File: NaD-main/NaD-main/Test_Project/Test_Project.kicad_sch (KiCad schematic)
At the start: 35 parts, among them J1 SWD, J2 USART1, J3 3V3, J5 Screw_Terminal_01x02, U1 AMS1117-3.3, U2 STM32F103C8Tx, U3 L298HN, U4 L7805, Y1 16 MHz

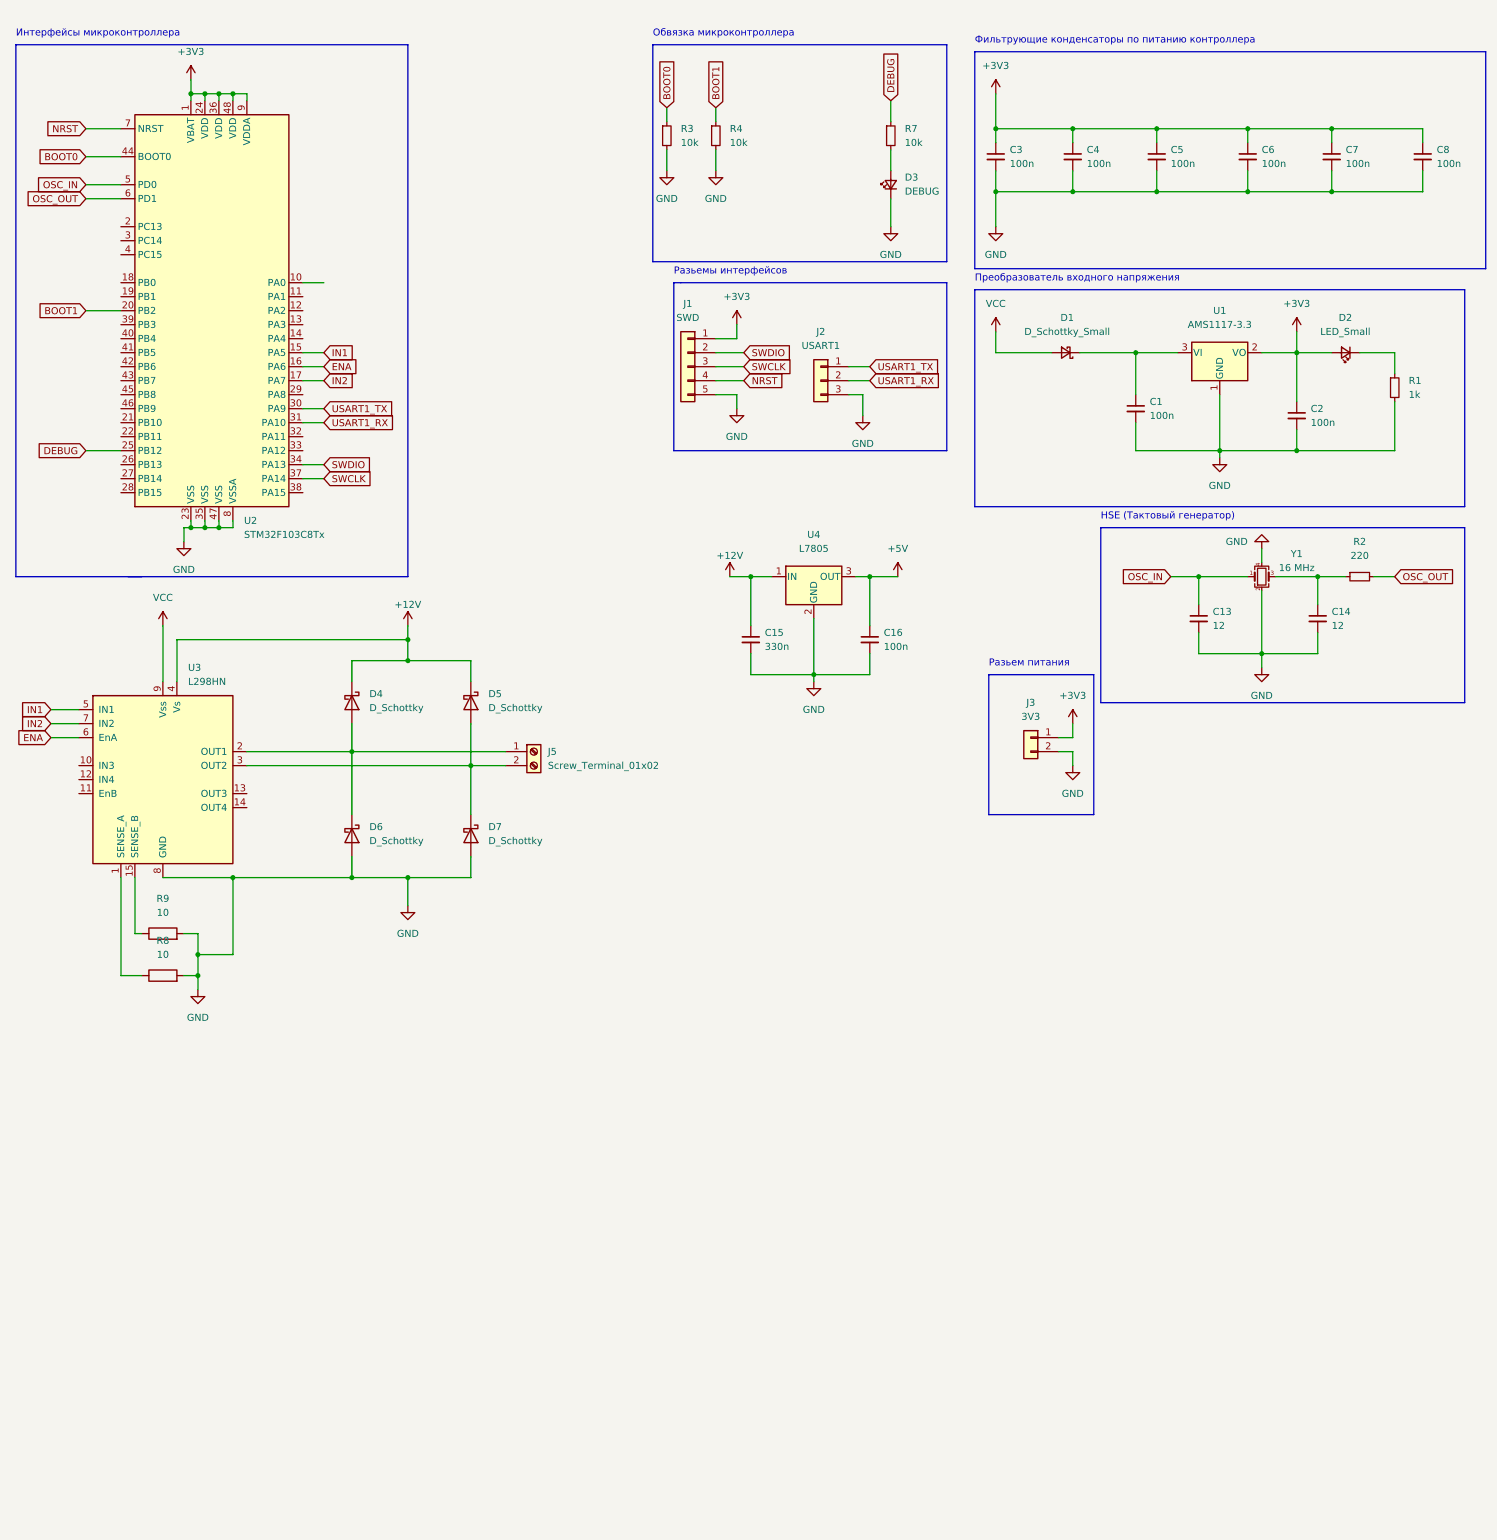
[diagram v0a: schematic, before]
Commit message: Documentation
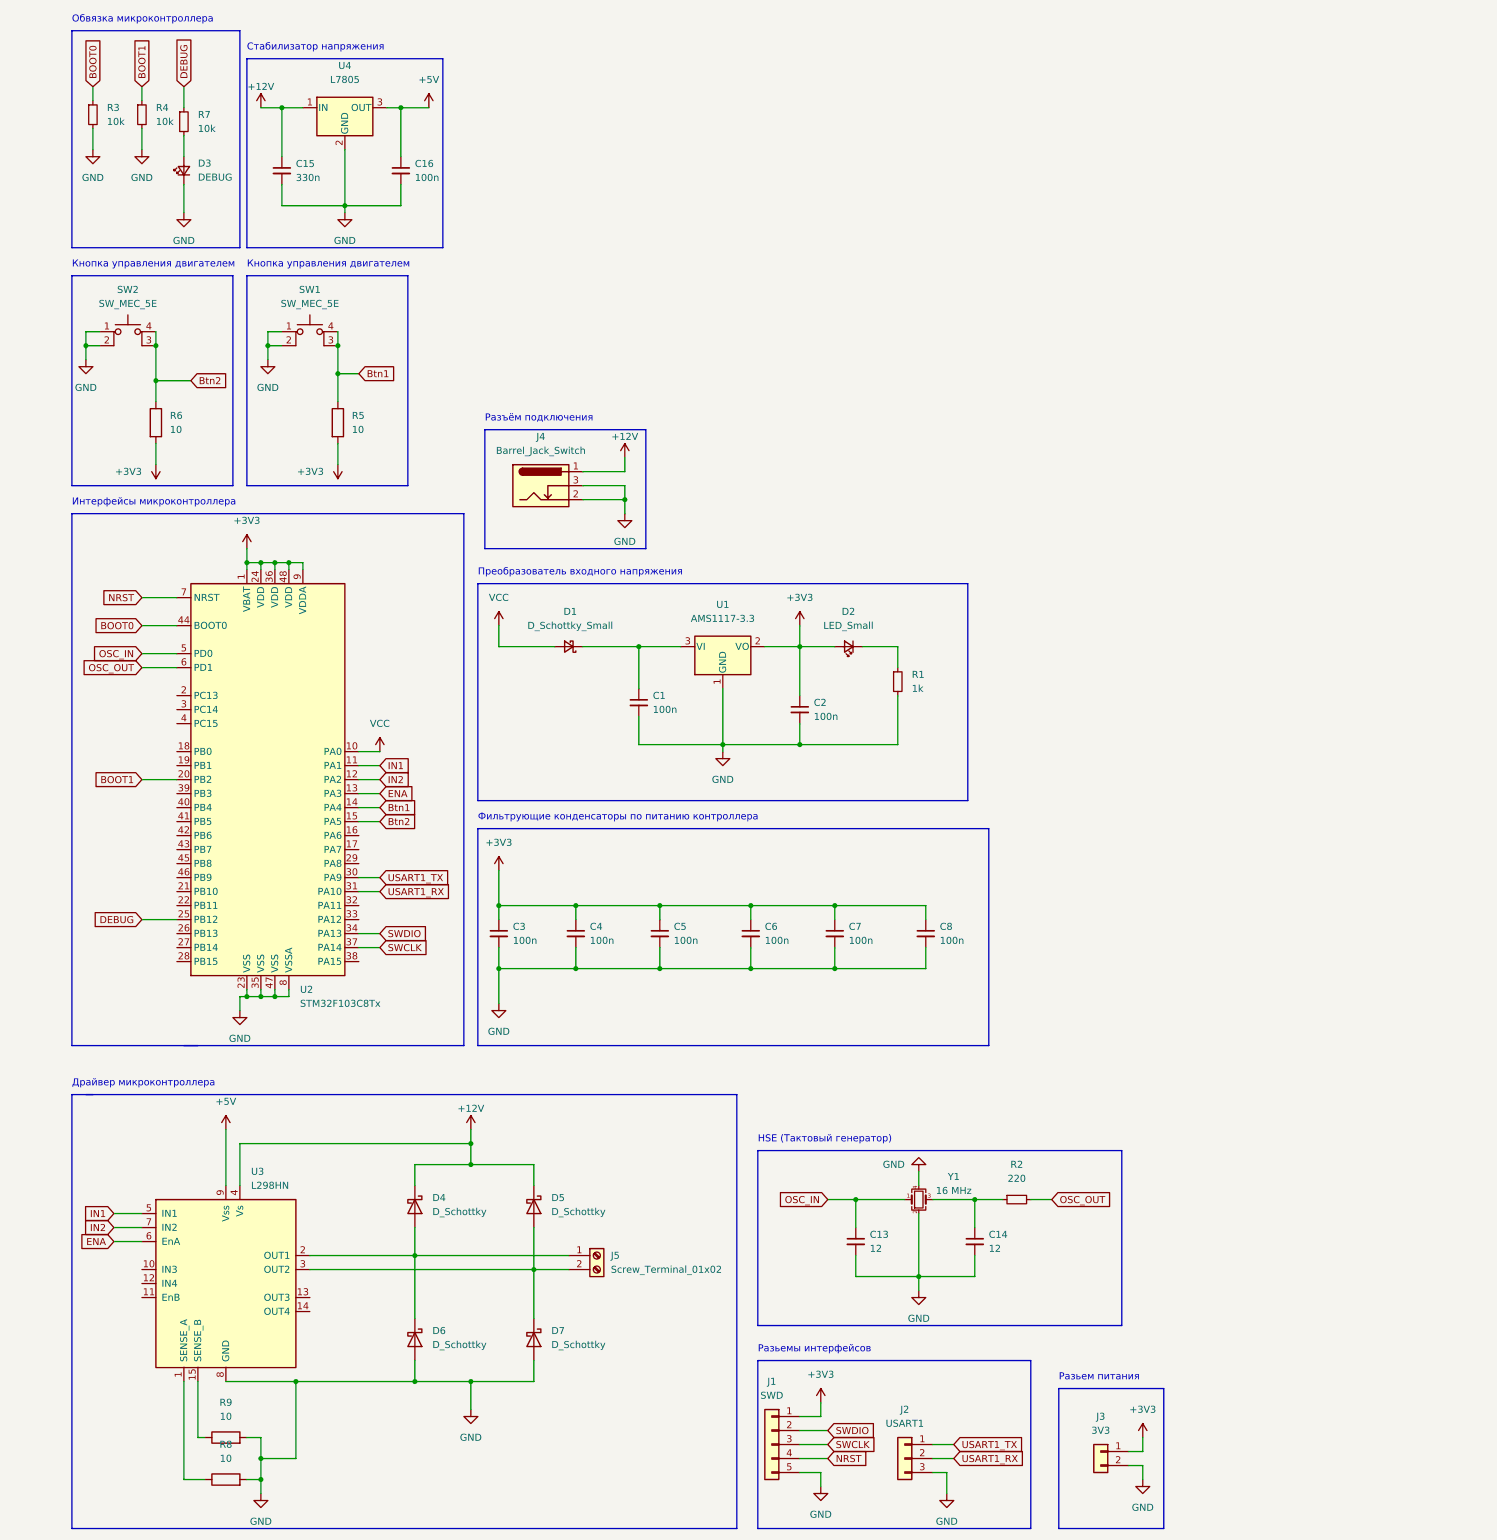
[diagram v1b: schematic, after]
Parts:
- added J4: Barrel_Jack_Switch, Connector_BarrelJack:BarrelJack_GCT_DCJ200-10-A_Horizontal, symbol Connector:Barrel_Jack_Switch
- added R5, R6: 10, Resistor_SMD:R_0805_2012Metric, symbol Device:R
- added SW1, SW2: SW_MEC_5E, CourseProject_Borisov:SW_PUSH_6mm, symbol Switch:SW_MEC_5E
- D4, D5, D6, D7: footprint Diode_SMD:D_0805_2012Metric -> Diode_SMD:D_SMA
- U3: footprint Package_TO_SOT_THT:TO-220-15_P2.54x2.54mm_StaggerOdd_Lead5.84mm_TabDown -> Package_TO_SOT_THT:TO-220-15_P2.54x2.54mm_StaggerOdd_Lead4.58mm_Vertical
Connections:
- net +12V: now also J4.1
- net +3V3: now also R5.2, R6.2
- net +5V: now also U3.9 (Vss)
- net ENA: now also U2.13 (PA3); no longer U2.16 (PA6)
- net GND: now also J4.2, J4.3, SW1.1, SW1.2, SW2.1, SW2.2
- net IN1: now also U2.11 (PA1); no longer U2.15 (PA5)
- net IN2: now also U2.12 (PA2); no longer U2.17 (PA7)
- net VCC: now also U2.10 (PA0); no longer U3.9 (Vss)
- net Btn1: now reaches U2.14 (PA4)
- net Btn1: now also R5.1, SW1.3 (K), SW1.4 (A)
- new net Btn2: R6.1, SW2.3 (K), SW2.4 (A), U2.15 (PA5)
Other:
- note added: "Драйвер микроконтроллера"
- note added: "Кнопка управления двигателем"
- note added: "Разъём подключения"
- note added: "Стабилизатор напряжения"
- company: (none) -> ВолгГту
- title: (none) -> Отладочная плата. Схема электронная принципиальная.
- moved on the sheet: C1, C13, C14, C15, C16, C2, C3, C4, C5, C6, C7, C8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
